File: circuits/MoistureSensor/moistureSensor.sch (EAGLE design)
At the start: 4 parts, among them P1 MCS10B, P2 MCS10B, Q1 BSS84

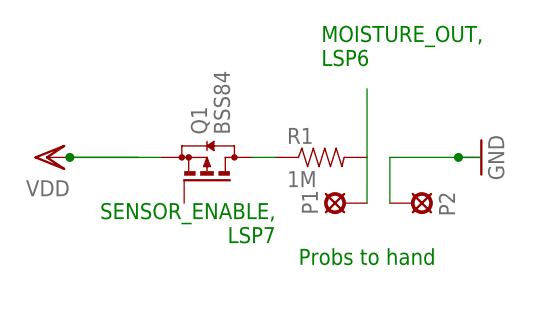
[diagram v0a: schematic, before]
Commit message: Moisture sesnsor layout final
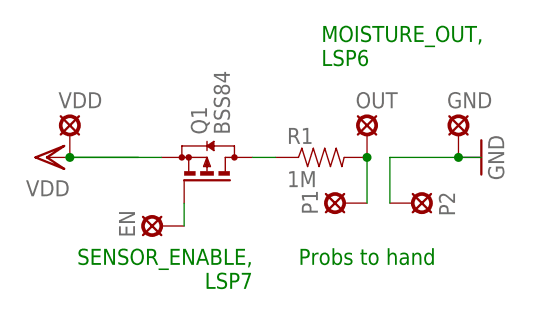
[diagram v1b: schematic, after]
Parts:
- added EN, GND, OUT, VDD: MCS10B, solpad:MCS10B
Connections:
- new net N$2: EN.MP, Q1.G
- net GND: now also GND.MP
- net N$3: now also OUT.MP
- net VDD: now also VDD.MP
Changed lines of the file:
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@@
 <grid distance="0.1" unitdist="inch" unit="inch" style="lines" multiple="1" display="no" altdistance="0.01" altunitdist="inch" altunit="inch"/>
 <layers>
-<layer number="1" name="Top" color="4" fill="1" visible="no" active="no"/>
-<layer number="16" name="Bottom" color="1" fill="1" visible="no" active="no"/>
-<layer number="17" name="Pads" color="2" fill="1" visible="no" active="no"/>
-<layer number="18" name="Vias" color="2" fill="1" visible="no" active="no"/>
-<layer number="19" name="Unrouted" color="6" fill="1" visible="no" active="no"/>
-<layer number="20" name="Dimension" color="15" fill="1" visible="no" active="no"/>
-<layer number="21" name="tPlace" color="7" fill="1" visible="no" active="no"/>
-<layer number="22" name="bPlace" color="7" fill="1" visible="no" active="no"/>
-<layer number="23" name="tOrigins" color="15" fill="1" visible="no" active="no"/>
-<layer number="24" name="bOrigins" color="15" fill="1" visible="no" active="no"/>
-<layer number="25" name="tNames" color="7" fill="1" visible="no" active="no"/>
-<layer number="26" name="bNames" color="7" fill="1" visible="no" active="no"/>
-<layer number="27" name="tValues" color="7" fill="1" visible="no" active="no"/>
-<layer number="28" name="bValues" color="7" fill="1" visible="no" active="no"/>
+<layer number="1" name="Top" color="4" fill="1" visible="yes" active="no"/>
+<layer number="16" name="Bottom" color="1" fill="1" visible="yes" active="no"/>
+<layer number="17" name="Pads" color="2" fill="1" visible="yes" active="no"/>
+<layer number="18" name="Vias" color="2" fill="1" visible="yes" active="no"/>
+<layer number="19" name="Unrouted" color="6" fill="1" visible="yes" active="no"/>
+<layer number="20" name="Dimension" color="15" fill="1" visible="yes" active="no"/>
+<layer number="21" name="tPlace" color="7" fill="1" visible="yes" active="no"/>
+<layer number="22" name="bPlace" color="7" fill="1" visible="yes" active="no"/>
+<layer number="23" name="tOrigins" color="15" fill="1" visible="yes" active="no"/>
+<layer number="24" name="bOrigins" color="15" fill="1" visible="yes" active="no"/>
+<layer number="25" name="tNames" color="7" fill="1" visible="yes" active="no"/>
+<layer number="26" name="bNames" color="7" fill="1" visible="yes" active="no"/>
+<layer number="27" name="tValues" color="7" fill="1" visible="yes" active="no"/>
+<layer number="28" name="bValues" color="7" fill="1" visible="yes" active="no"/>
 <layer number="29" name="tStop" color="7" fill="3" visible="no" active="no"/>
 <layer number="30" name="bStop" color="7" fill="6" visible="no" active="no"/>
@@
 <layer number="35" name="tGlue" color="7" fill="4" visible="no" active="no"/>
 <layer number="36" name="bGlue" color="7" fill="5" visible="no" active="no"/>
-<layer number="37" name="tTest" color="7" fill="1" visible="no" active="no"/>
-<layer number="38" name="bTest" color="7" fill="1" visible="no" active="no"/>
+<layer number="37" name="tTest" color="7" fill="1" visible="yes" active="no"/>
+<layer number="38" name="bTest" color="7" fill="1" visible="yes" active="no"/>
 <layer number="39" name="tKeepout" color="4" fill="11" visible="no" active="no"/>
 <layer number="40" name="bKeepout" color="1" fill="11" visible="no" active="no"/>
@@
 <layer number="44" name="Drills" color="7" fill="1" visible="no" active="no"/>
 <layer number="45" name="Holes" color="7" fill="1" visible="no" active="no"/>
-<layer number="46" name="Milling" color="3" fill="1" visible="no" active="no"/>
-<layer number="47" name="Measures" color="7" fill="1" visible="no" active="no"/>
-<layer number="48" name="Document" color="7" fill="1" visible="no" active="no"/>
-<layer number="49" name="Reference" color="13" fill="1" visible="no" active="no"/>
-<layer number="50" name="dxf" color="7" fill="1" visible="no" active="no"/>
-<layer number="51" name="tDocu" color="14" fill="1" visible="no" active="no"/>
-<layer number="52" name="bDocu" color="7" fill="1" visible="no" active="no"/>
-<layer number="53" name="tGND_GNDA" color="7" fill="9" visible="no" active="no"/>
-<layer number="54" name="bGND_GNDA" color="1" fill="9" visible="no" active="no"/>
-<layer number="56" name="wert" color="7" fill="1" visible="no" active="no"/>
-<layer number="57" name="tCAD" color="7" fill="1" visible="no" active="no"/>
+<layer number="46" name="Milling" color="3" fill="1" visible="yes" active="no"/>
+<layer number="47" name="Measures" color="7" fill="1" visible="yes" active="no"/>
+<layer number="48" name="Document" color="7" fill="1" visible="yes" active="no"/>
+<layer number="49" name="Reference" color="7" fill="1" visible="yes" active="no"/>
+<layer number="50" name="dxf" color="7" fill="1" visible="yes" active="no"/>
+<layer number="51" name="tDocu" color="7" fill="1" visible="yes" active="no"/>
+<layer number="52" name="bDocu" color="7" fill="1" visible="yes" active="no"/>
+<layer number="53" name="tGND_GNDA" color="7" fill="9" visible="yes" active="no"/>
+<layer number="54" name="bGND_GNDA" color="1" fill="9" visible="yes" active="no"/>
+<layer number="56" name="wert" color="7" fill="1" visible="yes" active="no"/>
+<layer number="57" name="tCAD" color="7" fill="1" visible="yes" active="no"/>
 <layer number="90" name="Modules" color="5" fill="1" visible="yes" active="yes"/>
 <layer number="91" name="Nets" color="2" fill="1" visible="yes" active="yes"/>
@@
 <part name="P1" library="solpad" deviceset="MCS10B" device=""/>
 <part name="P2" library="solpad" deviceset="MCS10B" device=""/>
+<part name="GND" library="solpad" deviceset="MCS10B" device=""/>
+<part name="VDD" library="solpad" deviceset="MCS10B" device=""/>
+<part name="EN" library="solpad" deviceset="MCS10B" device=""/>
+<part name="OUT" library="solpad" deviceset="MCS10B" device=""/>
 </parts>
 <sheets>
@@
 <text x="10.16" y="68.58" size="1.778" layer="91">MOISTURE_OUT,
 LSP6</text>
-<text x="5.08" y="53.34" size="1.778" layer="91" rot="R180">SENSOR_ENABLE,
+<text x="2.54" y="48.26" size="1.778" layer="91" rot="R180">SENSOR_ENABLE,
 LSP7</text>
 <text x="22.86" y="48.26" size="1.778" layer="91" rot="R180">Probs to hand</text>
@@
 <instance part="P1" gate="1" x="12.7" y="53.34" rot="R90"/>
 <instance part="P2" gate="1" x="20.32" y="53.34" rot="R270"/>
+<instance part="GND" gate="1" x="25.4" y="60.96"/>
+<instance part="VDD" gate="1" x="-17.78" y="60.96"/>
+<instance part="EN" gate="1" x="-7.62" y="50.8" rot="R90"/>
+<instance part="OUT" gate="1" x="15.24" y="60.96"/>
 </instances>
 <busses>
@@
 <segment>
 <pinref part="R1" gate="G$1" pin="2"/>
-<wire x1="15.24" y1="58.42" x2="15.24" y2="66.04" width="0.1524" layer="91"/>
 <pinref part="P1" gate="1" pin="MP"/>
 <wire x1="15.24" y1="58.42" x2="15.24" y2="53.34" width="0.1524" layer="91"/>
+<pinref part="OUT" gate="1" pin="MP"/>
+<junction x="15.24" y="58.42"/>
 </segment>
 </net>
@@
 <pinref part="P2" gate="1" pin="MP"/>
 <wire x1="17.78" y1="58.42" x2="17.78" y2="53.34" width="0.1524" layer="91"/>
+<pinref part="GND" gate="1" pin="MP"/>
 </segment>
 </net>
@@
 <junction x="-17.78" y="58.42"/>
 <wire x1="-17.78" y1="58.42" x2="-7.62" y2="58.42" width="0.1524" layer="91"/>
-</segment>
-</net>
+<pinref part="VDD" gate="1" pin="MP"/>
+</segment>
+</net>
+<net name="N$2" class="0">
+<segment>
+<pinref part="EN" gate="1" pin="MP"/>
+<pinref part="Q1" gate="G$1" pin="G"/>
+<wire x1="-5.08" y1="50.8" x2="-5.08" y2="53.34" width="0.1524" layer="91"/>
+</segment>
+</net>
